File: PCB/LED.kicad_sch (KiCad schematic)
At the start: 9 parts, among them Q2 2N7002

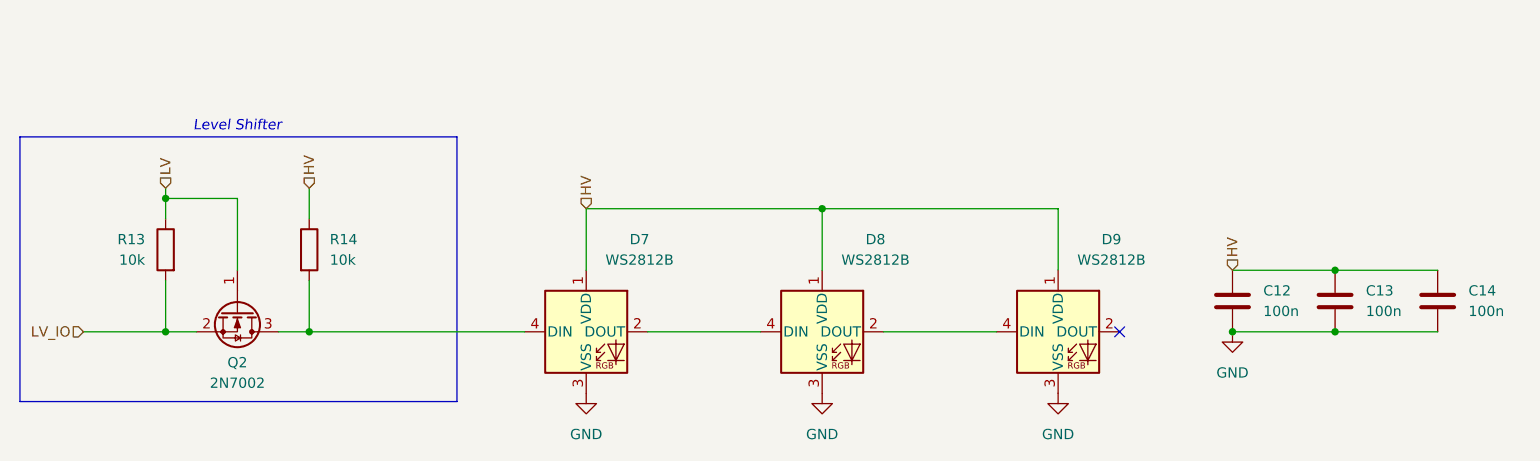
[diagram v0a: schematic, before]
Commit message: platformio commi
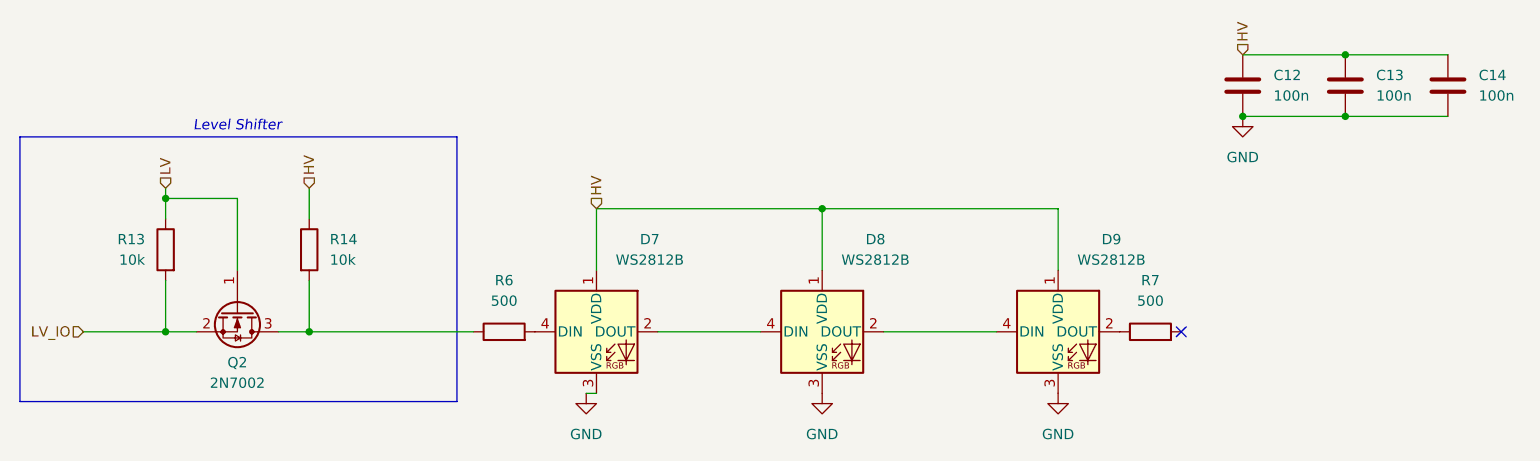
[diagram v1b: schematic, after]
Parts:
- added R6, R7: 500, Resistor_SMD:R_0402_1005Metric, symbol Device:R
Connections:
- net at Q2.3 (D), R14.2: now also R6.1; no longer D7.4 (DIN)
- net at D9.2 (DOUT): now also R7.1
- new net: D7.4 (DIN), R6.2
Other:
- moved on the sheet: C12, C13, C14, D7
